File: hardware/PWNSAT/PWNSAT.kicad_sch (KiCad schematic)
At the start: 0 parts

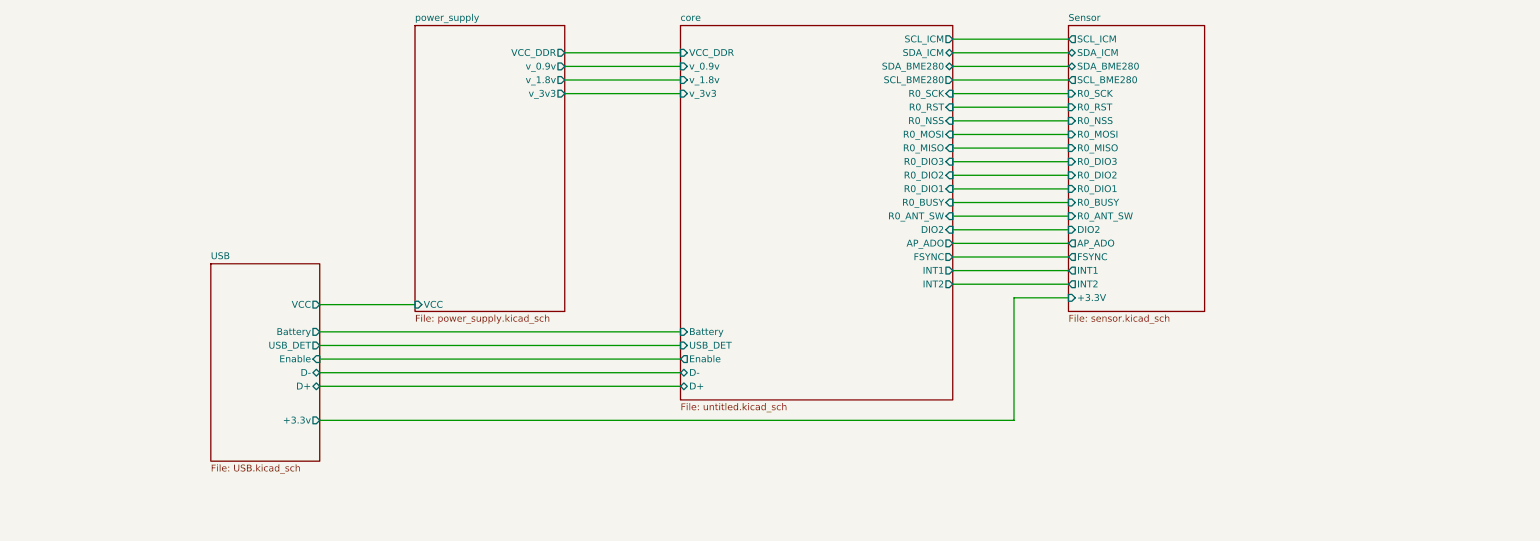
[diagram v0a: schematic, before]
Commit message: feat(Hw):Battery_Board_pro_Updated
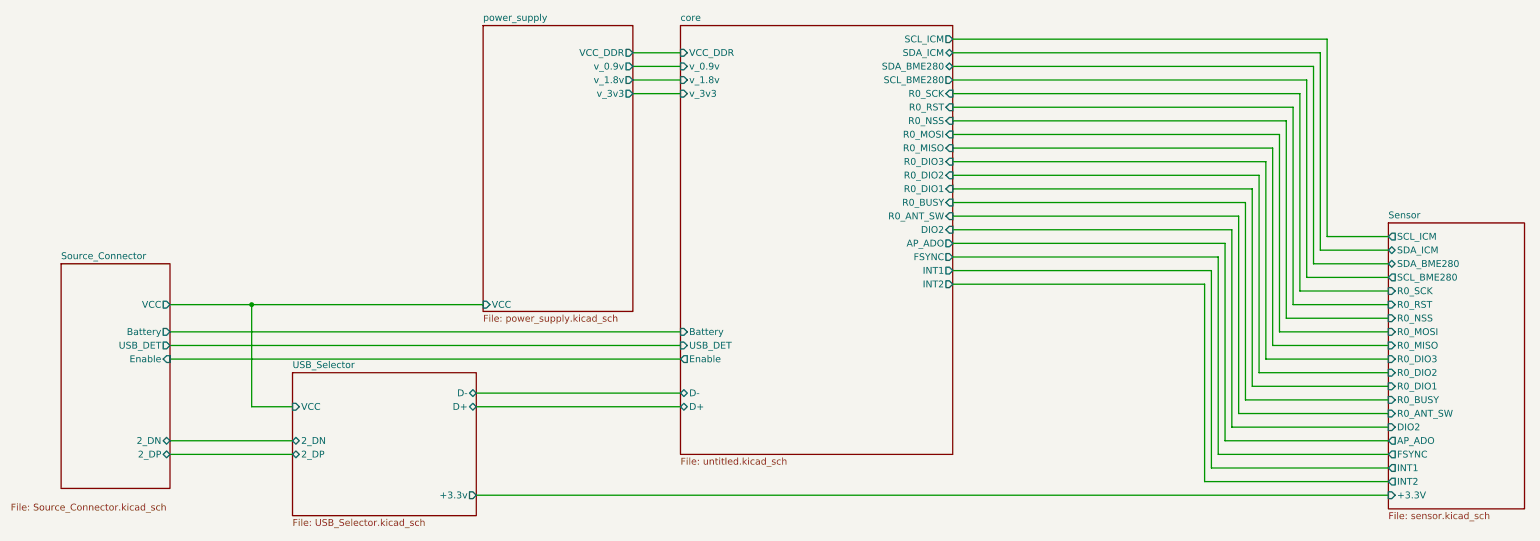
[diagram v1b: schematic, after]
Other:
- sheet USB renamed Source_Connector
- added sheet USB_Selector (USB_Selector.kicad_sch)
- sheet Source_Connector: file USB.kicad_sch -> Source_Connector.kicad_sch
- sheet Source_Connector ports: added 2_DN, 2_DP; removed +3.3v, D+, D-
